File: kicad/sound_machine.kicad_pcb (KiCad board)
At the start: 2 copper layers, 13 parts, among them J1 Conn_01x02, J2 Conn_01x15, J3 Conn_01x15, J4 TEST_1P, J5 Audio-Jack-3, J6 TEST_1P, J7 TEST_1P, J8 TEST_1P, U1 MPU-6050_breakout, U2 DFPlayerMini

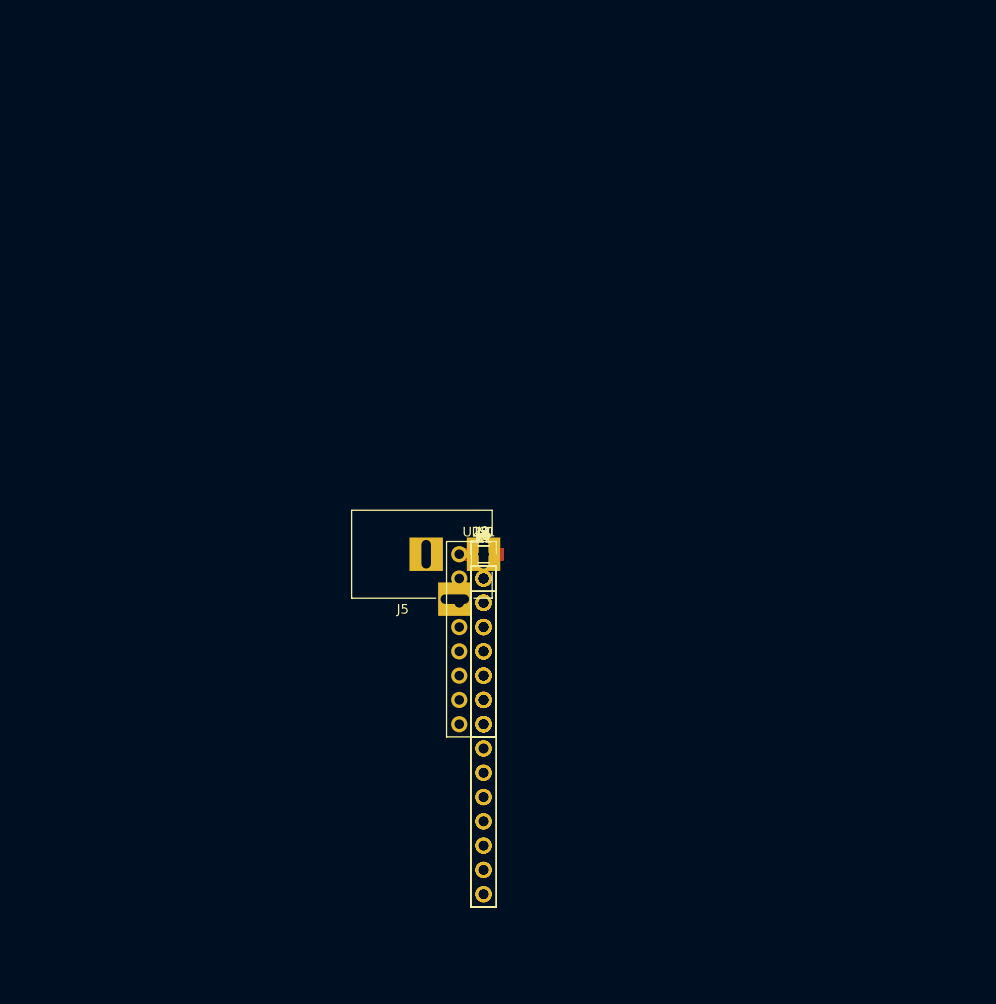
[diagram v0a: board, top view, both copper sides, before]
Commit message: Basic layout
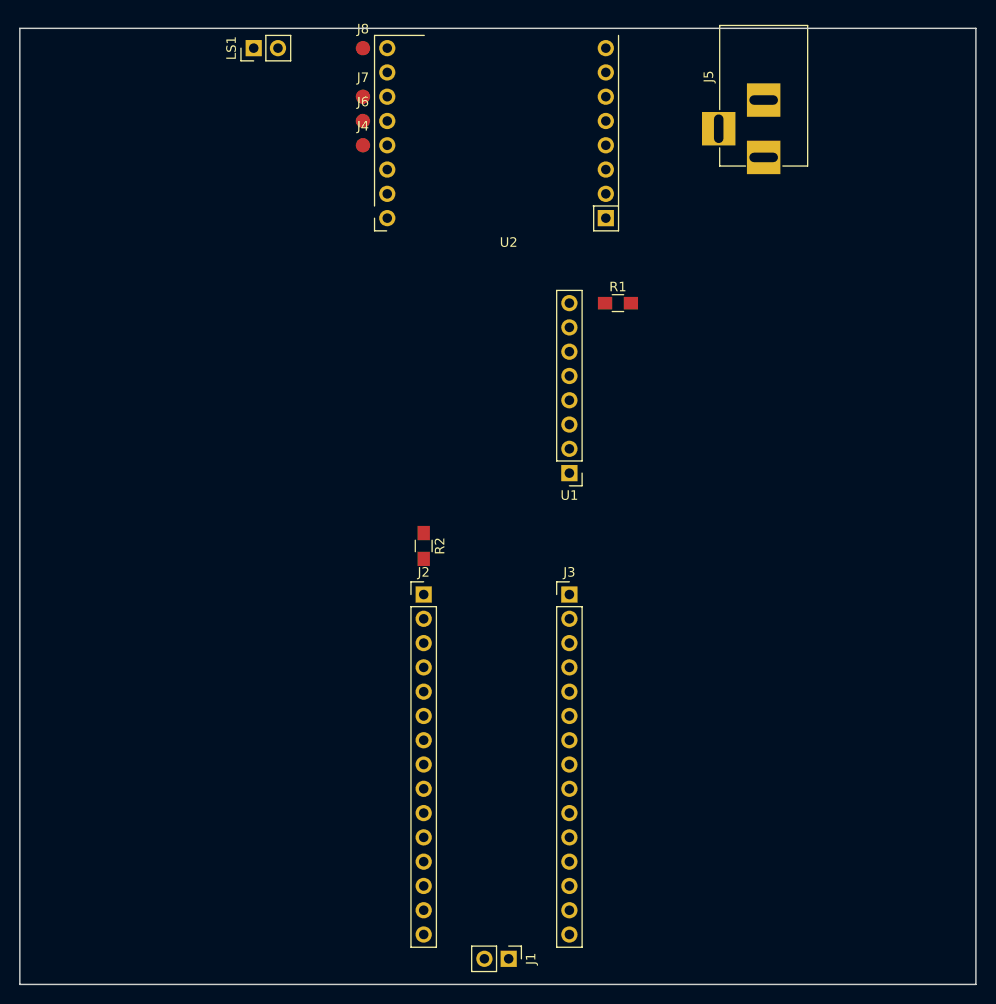
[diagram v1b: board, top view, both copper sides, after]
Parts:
- U2: footprint Socket_Strips:Socket_Strip_Straight_2x08_Pitch2.54mm -> DFPlayerMini
- moved LS1 58.1 mm to (124.5, 52.1), turned to 90 degrees
- moved J8 54.4 mm to (135.9, 52.1)
- moved J5 50.8 mm to (177.8, 63.5), turned to 270 degrees
- moved J7 49.5 mm to (135.9, 57.1)
- moved J6 47.0 mm to (135.9, 59.7)
- moved J4 44.6 mm to (135.9, 62.2)
- moved J1 42.4 mm to (151.1, 147.3), turned to 270 degrees
- moved U2 35.3 mm to (151.1, 69.8), turned to 180 degrees
- moved R1 29.8 mm to (162.6, 78.7)
- moved U1 12.4 mm to (157.5, 96.5), turned to 180 degrees
- moved J3 9.92 mm to (157.5, 109.2)
- moved J2 7.55 mm to (142.2, 109.2)
- moved R2 6.32 mm to (142.2, 104.1), turned to 270 degrees
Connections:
- U2 pad 10: Net-(U2-Pad10) -> GND
- U2 pad 11: Net-(U2-Pad11) -> Net-(J7-Pad1)
- U2 pad 12: Net-(J4-Pad1) -> Net-(J6-Pad1)
- U2 pad 13: Net-(J6-Pad1) -> Net-(J4-Pad1)
- U2 pad 14: Net-(J7-Pad1) -> Net-(U2-Pad14)
- U2 pad 15: GND -> Net-(U2-Pad15)
- U2 pad 16: Net-(J8-Pad1) -> Net-(U2-Pad16)
- U2 pad 9: Net-(U2-Pad9) -> Net-(J8-Pad1)
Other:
- board outline added: 100 x 100 mm
- net class Default: clearance 0.2 -> 0.1524; trace_width 0.25 -> 0.1524; via_dia 0.6 -> 0.6858; via_drill 0.4 -> 0.3302
- rule trace_clearance: 0.2 -> 0.1524
- rule trace_min: 0.2 -> 0.1524
- rule via_min_drill: 0.3 -> 0.3302
- rule via_min_size: 0.4 -> 0.6858
